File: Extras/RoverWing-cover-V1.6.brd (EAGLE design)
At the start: 81.3 x 81.3 mm, 52 parts, among them J1 HEADER-PH-3PSIDEENTRY, J10 HEADER-PH-6PSIDEENTRY, J13 HEADER-PH-6PSIDEENTRY, J16 FEATHERWING_NODIM, J17 HEADER-PH-6PSIDEENTRY, J5 HEADER-PH-6PSIDEENTRY

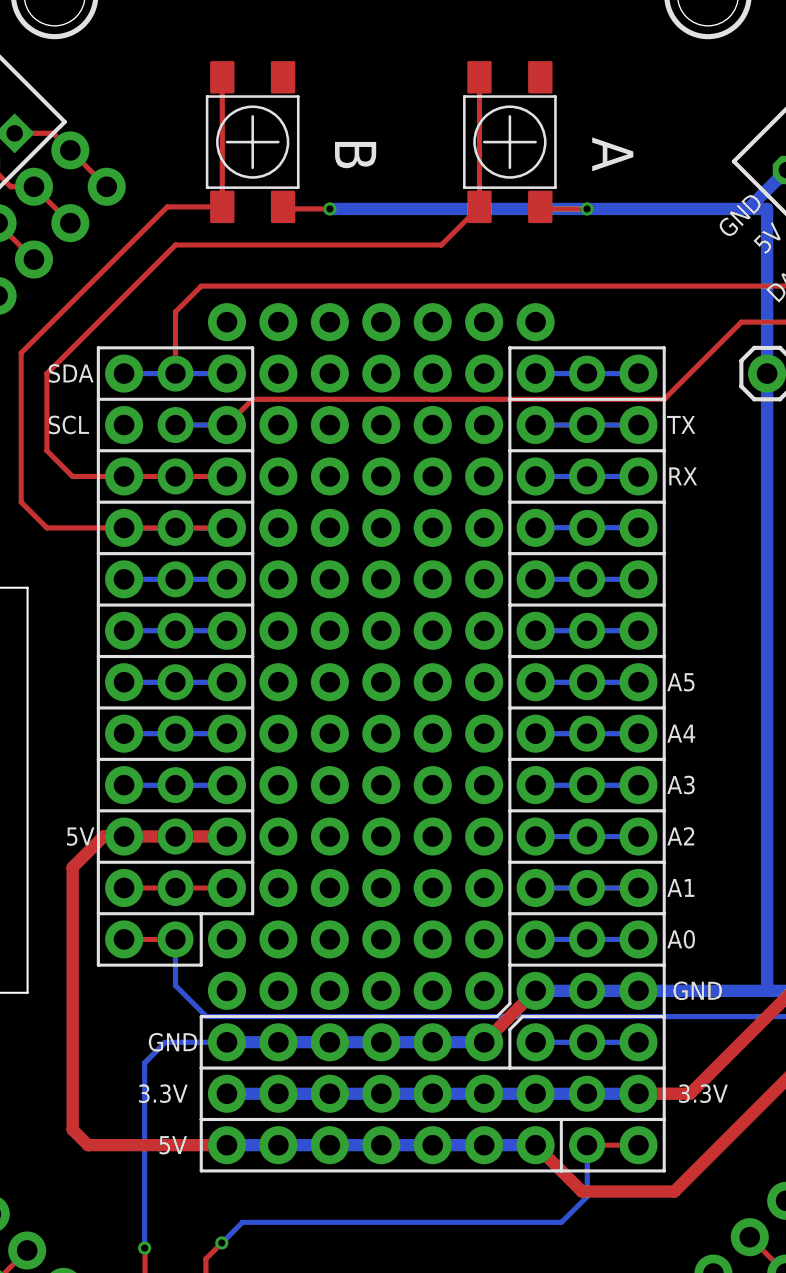
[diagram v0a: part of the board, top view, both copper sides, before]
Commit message: Update RoverWing-cover-V1.6.brd
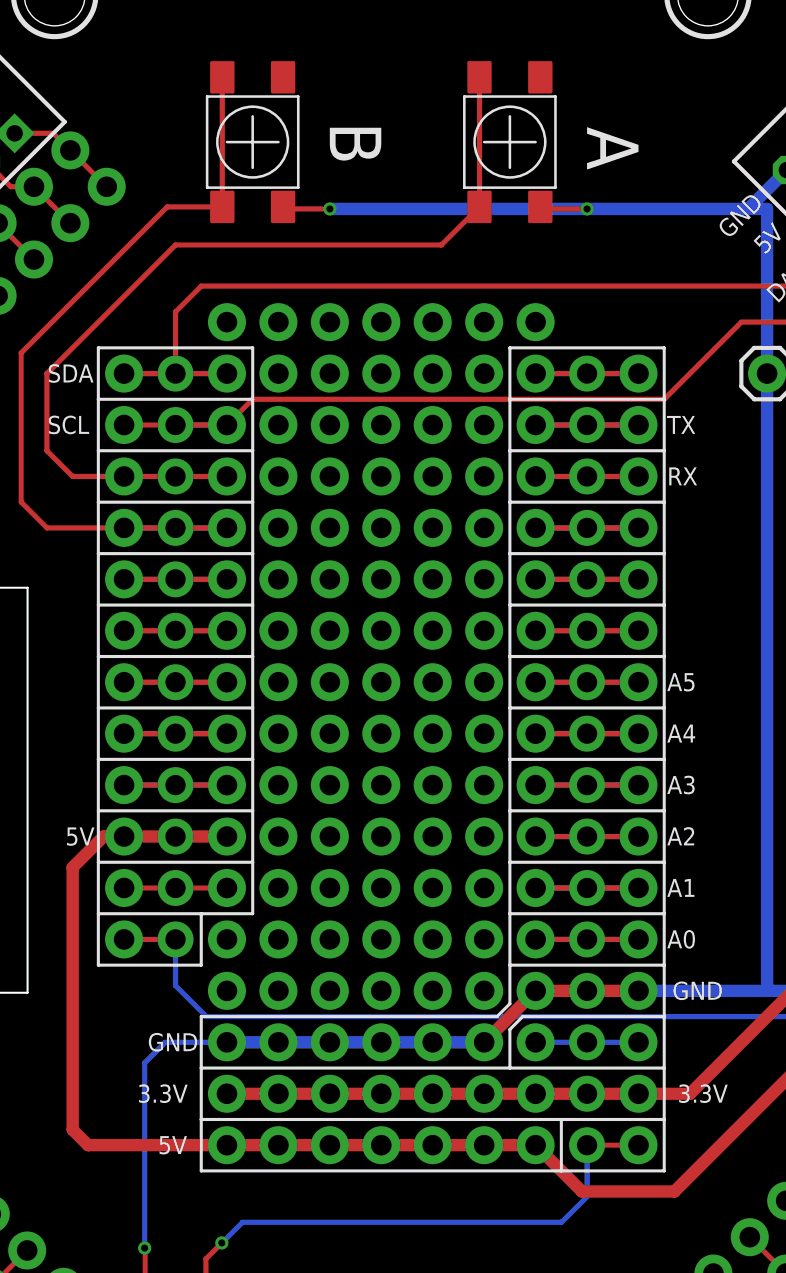
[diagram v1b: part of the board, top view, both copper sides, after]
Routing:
- net TX: track 5.08 -> 10.4 mm
- net SCK: track 5.08 -> 10.2 mm
- net RX: track 5.08 -> 10.2 mm
- net MOSI: track 5.08 -> 10.2 mm
- net MISO: track 5.08 -> 10.2 mm
- net EXTRA: track 5.08 -> 10.2 mm
- net D13: track 5.08 -> 10.2 mm
- net D12: track 5.08 -> 10.2 mm
- net D11: track 5.08 -> 10.2 mm
- net D10: track 5.08 -> 10.2 mm
- net D09: track 5.08 -> 10.2 mm
- net A5: track 5.08 -> 10.2 mm
- net A4: track 5.08 -> 10.2 mm
- net A3: track 5.08 -> 10.2 mm
- net A2: track 5.08 -> 10.2 mm
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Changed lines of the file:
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@@
 <wire x1="6.35" y1="15.24" x2="13.97" y2="15.24" width="0.1524" layer="22"/>
 <wire x1="6.35" y1="17.78" x2="13.97" y2="17.78" width="0.1524" layer="22"/>
-<text x="10.414" y="30.734" size="2.032" layer="25" font="vector" ratio="14" rot="SR270">A</text>
-<text x="-2.286" y="30.734" size="2.032" layer="25" font="vector" ratio="14" rot="SR270">B</text>
+<text x="10.16" y="31.242" size="2.54" layer="25" font="vector" ratio="14" rot="SR270">A</text>
+<text x="-2.54" y="31.496" size="2.54" layer="25" font="vector" ratio="14" rot="SR270">B</text>
 <wire x1="-8.89" y1="-7.62" x2="-8.89" y2="-10.16" width="0.1524" layer="21"/>
 <wire x1="-13.97" y1="-10.16" x2="-8.89" y2="-10.16" width="0.1524" layer="22"/>
@@
 <contactref element="S3" pad="2"/>
 <wire x1="-7.62" y1="-13.97" x2="5.08" y2="-13.97" width="0.6096" layer="16"/>
-<wire x1="7.62" y1="-11.43" x2="12.7" y2="-11.43" width="0.6096" layer="16"/>
 <wire x1="10.16" y1="27.178" x2="-2.54" y2="27.178" width="0.6096" layer="16"/>
 <via x="-2.54" y="27.178" extent="1-16" drill="0.35"/>
@@
 <wire x1="34.685" y1="-1.75" x2="32.484" y2="-1.75" width="0.3048" layer="1"/>
 <wire x1="32.484" y1="-1.75" x2="31.623" y2="-0.889" width="0.3048" layer="1"/>
+<wire x1="7.62" y1="-11.43" x2="12.7" y2="-11.43" width="0.6096" layer="1"/>
 <wire x1="-11.66" y1="-27.28" x2="-11.66" y2="-33.68" width="0" layer="19" extent="1-1"/>
 <wire x1="29.337" y1="-8.509" x2="29.21" y2="-8.509" width="0" layer="19" extent="1-16"/>
@@
 <wire x1="26.543" y1="28.829" x2="22.584209375" y2="28.829" width="0.6096" layer="1"/>
 <wire x1="21.441209375" y1="27.686" x2="22.584209375" y2="28.829" width="0.6096" layer="1"/>
-<wire x1="-7.62" y1="-19.05" x2="7.62" y2="-19.05" width="0.6096" layer="16"/>
 <wire x1="34.544" y1="-14.224" x2="38.862" y2="-9.906" width="0.6096" layer="1"/>
 <wire x1="38.862" y1="-9.906" x2="38.862" y2="-7.62" width="0.6096" layer="1"/>
@@
 <wire x1="36.435" y1="-5.87" x2="36.435" y2="-7.507" width="0.3048" layer="1"/>
 <wire x1="36.435" y1="-7.507" x2="36.322" y2="-7.62" width="0.3048" layer="1"/>
+<wire x1="7.62" y1="-19.05" x2="-7.62" y2="-19.05" width="0.6096" layer="1"/>
 <wire x1="-2.54" y1="-19.05" x2="-5.08" y2="-19.05" width="0" layer="19" extent="1-1"/>
 <wire x1="0" y1="-19.05" x2="-2.54" y2="-19.05" width="0" layer="19" extent="1-1"/>
@@
 <contactref element="J113" pad="7"/>
 <wire x1="10.16" y1="-8.89" x2="7.62" y2="-8.89" width="0.254" layer="16"/>
+<wire x1="7.62" y1="-8.89" x2="12.7" y2="-8.89" width="0.254" layer="1"/>
 </signal>
 <signal name="A1">
@@
 <wire x1="12.7" y1="-6.35" x2="10.16" y2="-6.35" width="0.254" layer="16"/>
 <wire x1="10.16" y1="-6.35" x2="7.62" y2="-6.35" width="0.254" layer="16"/>
+<wire x1="7.62" y1="-6.35" x2="12.7" y2="-6.35" width="0.254" layer="1"/>
 </signal>
 <signal name="A2">
@@
 <wire x1="12.7" y1="-3.81" x2="10.16" y2="-3.81" width="0.254" layer="16"/>
 <wire x1="10.16" y1="-3.81" x2="7.62" y2="-3.81" width="0.254" layer="16"/>
+<wire x1="7.62" y1="-3.81" x2="12.7" y2="-3.81" width="0.254" layer="1"/>
 </signal>
 <signal name="A3">
@@
 <wire x1="12.7" y1="-1.27" x2="10.16" y2="-1.27" width="0.254" layer="16"/>
 <wire x1="10.16" y1="-1.27" x2="7.62" y2="-1.27" width="0.254" layer="16"/>
+<wire x1="7.62" y1="-1.27" x2="12.7" y2="-1.27" width="0.254" layer="1"/>
 </signal>
 <signal name="A4">
@@
 <wire x1="12.7" y1="1.27" x2="10.16" y2="1.27" width="0.254" layer="16"/>
 <wire x1="10.16" y1="1.27" x2="7.62" y2="1.27" width="0.254" layer="16"/>
+<wire x1="7.62" y1="1.27" x2="12.7" y2="1.27" width="0.254" layer="1"/>
 </signal>
 <signal name="A5">
@@
 <wire x1="12.7" y1="3.81" x2="10.16" y2="3.81" width="0.254" layer="16"/>
 <wire x1="10.16" y1="3.81" x2="7.62" y2="3.81" width="0.254" layer="16"/>
+<wire x1="7.62" y1="3.81" x2="12.7" y2="3.81" width="0.254" layer="1"/>
 </signal>
 <signal name="SCK">
@@
 <wire x1="7.62" y1="6.35" x2="10.16" y2="6.35" width="0.254" layer="16"/>
 <wire x1="10.16" y1="6.35" x2="12.7" y2="6.35" width="0.254" layer="16"/>
+<wire x1="7.62" y1="6.35" x2="12.7" y2="6.35" width="0.254" layer="1"/>
 </signal>
 <signal name="MOSI">
@@
 <wire x1="7.62" y1="8.89" x2="10.16" y2="8.89" width="0.254" layer="16"/>
 <wire x1="10.16" y1="8.89" x2="12.7" y2="8.89" width="0.254" layer="16"/>
+<wire x1="7.62" y1="8.89" x2="12.7" y2="8.89" width="0.254" layer="1"/>
 </signal>
 <signal name="MISO">
@@
 <wire x1="7.62" y1="11.43" x2="10.16" y2="11.43" width="0.254" layer="16"/>
 <wire x1="12.7" y1="11.43" x2="10.16" y2="11.43" width="0.254" layer="16"/>
+<wire x1="7.62" y1="11.43" x2="12.7" y2="11.43" width="0.254" layer="1"/>
 </signal>
 <signal name="RX">
@@
 <wire x1="12.7" y1="13.97" x2="10.16" y2="13.97" width="0.254" layer="16"/>
 <wire x1="10.16" y1="13.97" x2="7.62" y2="13.97" width="0.254" layer="16"/>
+<wire x1="7.62" y1="13.97" x2="12.7" y2="13.97" width="0.254" layer="1"/>
 </signal>
 <signal name="TX">
@@
 <wire x1="12.7" y1="16.51" x2="10.16" y2="16.51" width="0.254" layer="16"/>
 <wire x1="10.16" y1="16.51" x2="7.62" y2="16.51" width="0.254" layer="16"/>
+<wire x1="7.62" y1="16.51" x2="12.954" y2="16.51" width="0.254" layer="1"/>
 </signal>
 <signal name="EXTRA">
@@
 <wire x1="10.16" y1="19.05" x2="7.62" y2="19.05" width="0.254" layer="16"/>
 <wire x1="12.7" y1="19.05" x2="10.16" y2="19.05" width="0.254" layer="16"/>
+<wire x1="7.62" y1="19.05" x2="12.7" y2="19.05" width="0.254" layer="1"/>
 </signal>
 <signal name="N$37">
@@
 <wire x1="-12.7" y1="-1.27" x2="-10.16" y2="-1.27" width="0.254" layer="16"/>
 <wire x1="-10.16" y1="-1.27" x2="-7.62" y2="-1.27" width="0.254" layer="16"/>
+<wire x1="-12.7" y1="-1.27" x2="-7.62" y2="-1.27" width="0.254" layer="1"/>
 </signal>
 <signal name="D12">
@@
 <wire x1="-12.7" y1="1.27" x2="-10.16" y2="1.27" width="0.254" layer="16"/>
 <wire x1="-10.16" y1="1.27" x2="-7.62" y2="1.27" width="0.254" layer="16"/>
+<wire x1="-12.7" y1="1.27" x2="-7.62" y2="1.27" width="0.254" layer="1"/>
 </signal>
 <signal name="D11">
@@
 <wire x1="-12.7" y1="3.81" x2="-10.16" y2="3.81" width="0.254" layer="16"/>
 <wire x1="-10.16" y1="3.81" x2="-7.62" y2="3.81" width="0.254" layer="16"/>
+<wire x1="-12.7" y1="3.81" x2="-7.62" y2="3.81" width="0.254" layer="1"/>
 </signal>
 <signal name="D10">
@@
 <wire x1="-12.7" y1="6.35" x2="-10.16" y2="6.35" width="0.254" layer="16"/>
 <wire x1="-10.16" y1="6.35" x2="-7.62" y2="6.35" width="0.254" layer="16"/>
+<wire x1="-12.7" y1="6.35" x2="-7.62" y2="6.35" width="0.254" layer="1"/>
 </signal>
 <signal name="D06">
@@
 <wire x1="-12.7" y1="8.89" x2="-10.16" y2="8.89" width="0.254" layer="16"/>
 <wire x1="-10.16" y1="8.89" x2="-7.62" y2="8.89" width="0.254" layer="16"/>
+<wire x1="-12.7" y1="8.89" x2="-7.62" y2="8.89" width="0.254" layer="1"/>
 </signal>
 <signal name="N$3">
@@
 <wire x1="26.67" y1="19.05" x2="22.352" y2="23.368" width="0.254" layer="1"/>
 <wire x1="-8.89" y1="23.368" x2="22.352" y2="23.368" width="0.254" layer="1"/>
+<wire x1="-12.7" y1="19.05" x2="-7.62" y2="19.05" width="0.254" layer="1"/>
 </signal>
 <signal name="SCL">
@@
 <wire x1="17.78" y1="21.59" x2="21.59" y2="21.59" width="0.254" layer="1"/>
 <wire x1="21.59" y1="21.59" x2="24.13" y2="19.05" width="0.254" layer="1"/>
-<wire x1="-12.7" y1="16.51" x2="-10.16" y2="16.51" width="0" layer="19" extent="1-1"/>
+<wire x1="-12.7" y1="16.51" x2="-7.62" y2="16.51" width="0.254" layer="1"/>
 </signal>
 <signal name="3.3V">
@@
 <contactref element="J116" pad="1"/>
 <contactref element="J2" pad="2"/>
-<wire x1="-7.62" y1="-16.51" x2="12.7" y2="-16.51" width="0.6096" layer="16"/>
 <wire x1="21.59" y1="19.05" x2="21.59" y2="-10.16" width="0.6096" layer="1"/>
 <wire x1="21.59" y1="-10.16" x2="15.24" y2="-16.51" width="0.6096" layer="1"/>
 <wire x1="15.24" y1="-16.51" x2="12.7" y2="-16.51" width="0.6096" layer="1"/>
+<wire x1="-7.62" y1="-16.51" x2="12.7" y2="-16.51" width="0.6096" layer="1"/>
 <wire x1="-2.54" y1="-16.51" x2="-5.08" y2="-16.51" width="0" layer="19" extent="1-1"/>
 <wire x1="0" y1="-16.51" x2="-2.54" y2="-16.51" width="0" layer="19" extent="1-1"/>

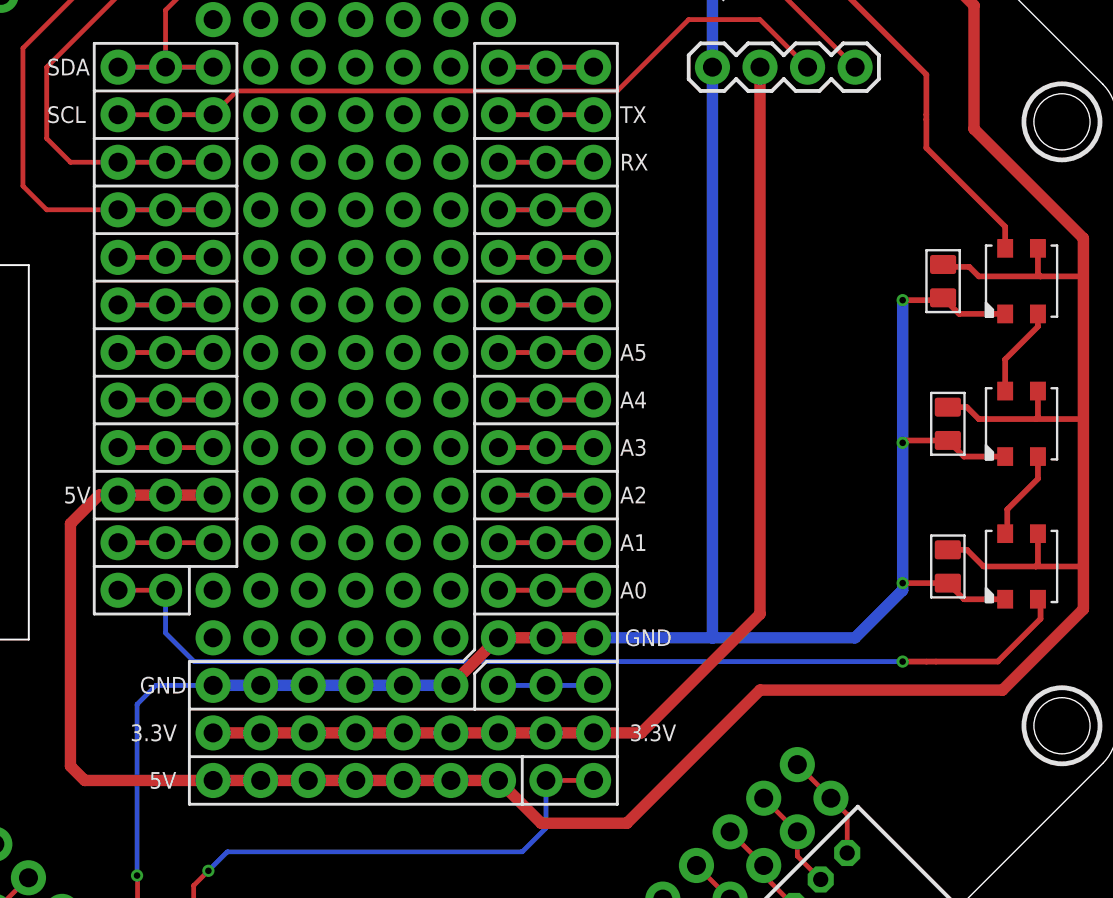
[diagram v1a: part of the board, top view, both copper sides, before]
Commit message: docs update
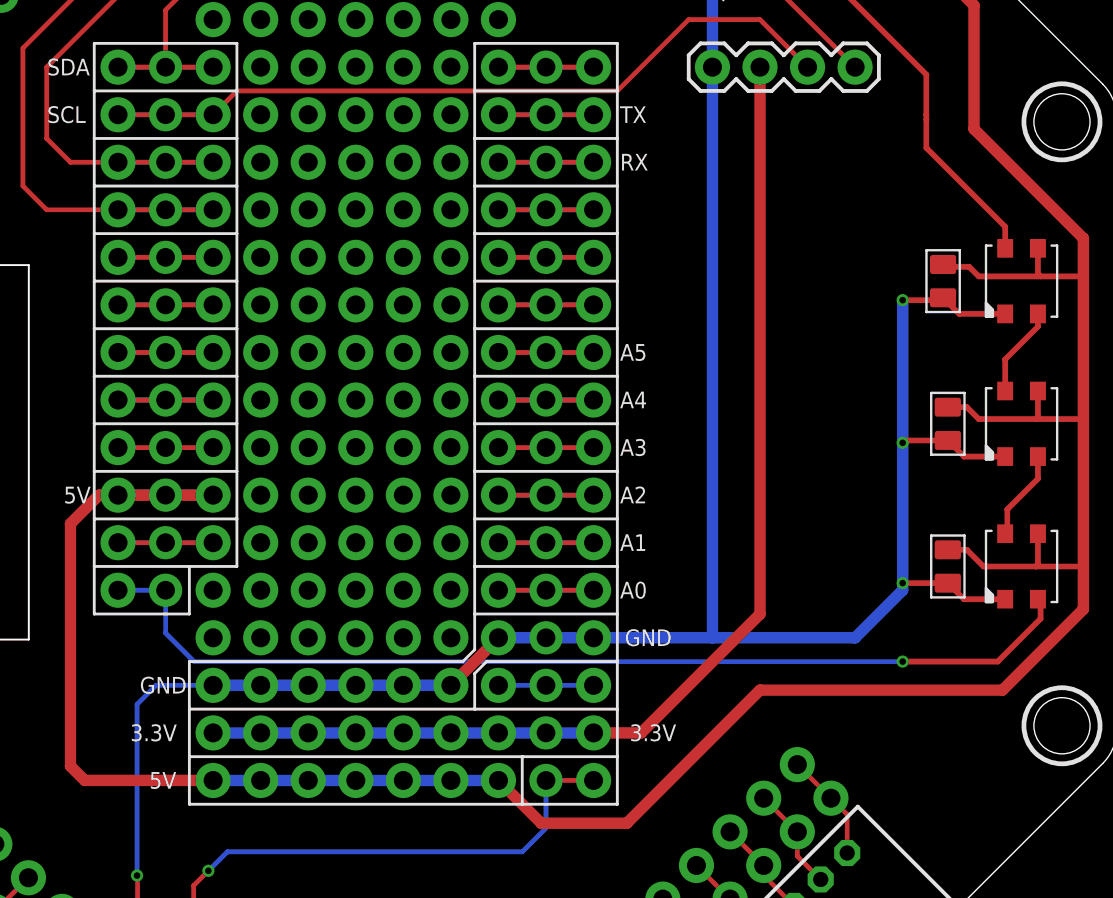
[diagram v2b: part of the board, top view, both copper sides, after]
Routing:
- net 5V: track 158.5 -> 163.6 mm
- net N$37: track 5.08 -> 10.2 mm
- net SCL: track 42.5 -> 45.1 mm
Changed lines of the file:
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@@
 <contactref element="S3" pad="3"/>
 <contactref element="S3" pad="2"/>
-<wire x1="-7.62" y1="-13.97" x2="5.08" y2="-13.97" width="0.6096" layer="16"/>
 <wire x1="10.16" y1="27.178" x2="-2.54" y2="27.178" width="0.6096" layer="16"/>
 <via x="-2.54" y="27.178" extent="1-16" drill="0.35"/>
@@
 <wire x1="34.685" y1="-1.75" x2="32.484" y2="-1.75" width="0.3048" layer="1"/>
 <wire x1="32.484" y1="-1.75" x2="31.623" y2="-0.889" width="0.3048" layer="1"/>
-<wire x1="7.62" y1="-11.43" x2="12.7" y2="-11.43" width="0.6096" layer="1"/>
+<wire x1="-7.62" y1="-13.97" x2="5.08" y2="-13.97" width="0.6096" layer="16"/>
+<wire x1="12.7" y1="-11.43" x2="7.62" y2="-11.43" width="0.6096" layer="16"/>
 <wire x1="-11.66" y1="-27.28" x2="-11.66" y2="-33.68" width="0" layer="19" extent="1-1"/>
 <wire x1="29.337" y1="-8.509" x2="29.21" y2="-8.509" width="0" layer="19" extent="1-16"/>
@@
 <wire x1="0" y1="-13.97" x2="-2.54" y2="-13.97" width="0" layer="19" extent="1-1"/>
 <wire x1="2.54" y1="-13.97" x2="5.08" y2="-13.97" width="0" layer="19" extent="16-16"/>
-<wire x1="10.16" y1="-11.43" x2="7.62" y2="-11.43" width="0" layer="19" extent="1-1"/>
+<wire x1="10.16" y1="-11.43" x2="12.7" y2="-11.43" width="0" layer="19" extent="1-1"/>
 <wire x1="7.85" y1="33.68" x2="7.85" y2="27.28" width="0" layer="19" extent="1-1"/>
 <wire x1="-4.85" y1="33.68" x2="-4.85" y2="27.28" width="0" layer="19" extent="1-1"/>
@@
 <wire x1="36.435" y1="-5.87" x2="36.435" y2="-7.507" width="0.3048" layer="1"/>
 <wire x1="36.435" y1="-7.507" x2="36.322" y2="-7.62" width="0.3048" layer="1"/>
-<wire x1="7.62" y1="-19.05" x2="-7.62" y2="-19.05" width="0.6096" layer="1"/>
+<wire x1="-7.62" y1="-19.05" x2="7.62" y2="-19.05" width="0.6096" layer="16"/>
+<wire x1="-12.7" y1="-3.81" x2="-7.62" y2="-3.81" width="0.6096" layer="16"/>
 <wire x1="-2.54" y1="-19.05" x2="-5.08" y2="-19.05" width="0" layer="19" extent="1-1"/>
 <wire x1="0" y1="-19.05" x2="-2.54" y2="-19.05" width="0" layer="19" extent="1-1"/>
@@
 <contactref element="J112" pad="1"/>
 <wire x1="-10.16" y1="-6.35" x2="-7.62" y2="-6.35" width="0.254" layer="1"/>
+<wire x1="-12.7" y1="-6.35" x2="-7.62" y2="-6.35" width="0.254" layer="16"/>
 </signal>
 <signal name="D13">
@@
 <wire x1="21.59" y1="21.59" x2="24.13" y2="19.05" width="0.254" layer="1"/>
 <wire x1="-12.7" y1="16.51" x2="-7.62" y2="16.51" width="0.254" layer="1"/>
+<wire x1="-12.7" y1="16.51" x2="-10.16" y2="16.51" width="0.254" layer="16"/>
 </signal>
 <signal name="3.3V">
@@
 <wire x1="21.59" y1="-10.16" x2="15.24" y2="-16.51" width="0.6096" layer="1"/>
 <wire x1="15.24" y1="-16.51" x2="12.7" y2="-16.51" width="0.6096" layer="1"/>
-<wire x1="-7.62" y1="-16.51" x2="12.7" y2="-16.51" width="0.6096" layer="1"/>
+<wire x1="-7.62" y1="-16.51" x2="12.7" y2="-16.51" width="0.6096" layer="16"/>
 <wire x1="-2.54" y1="-16.51" x2="-5.08" y2="-16.51" width="0" layer="19" extent="1-1"/>
 <wire x1="0" y1="-16.51" x2="-2.54" y2="-16.51" width="0" layer="19" extent="1-1"/>
@@
 <contactref element="J16" pad="28"/>
 <contactref element="J3" pad="1"/>
-<wire x1="-12.7" y1="-8.89" x2="-10.16" y2="-8.89" width="0.254" layer="1"/>
 <wire x1="-8.636" y1="-12.7" x2="-10.16" y2="-11.176" width="0.254" layer="16"/>
 <wire x1="-10.16" y1="-8.89" x2="-10.16" y2="-11.176" width="0.254" layer="16"/>
 <wire x1="-8.636" y1="-12.7" x2="29.21" y2="-12.7" width="0.254" layer="16"/>
 <via x="29.21" y="-12.7" extent="1-16" drill="0.35"/>
-<wire x1="29.21" y1="-12.7" x2="30.48" y2="-12.7" width="0.3048" layer="1"/>
-<wire x1="30.48" y1="-12.7" x2="30.988" y2="-12.7" width="0.3048" layer="1"/>
-<wire x1="30.988" y1="-12.7" x2="34.29" y2="-12.7" width="0.3048" layer="1"/>
+<wire x1="29.21" y1="-12.7" x2="34.29" y2="-12.7" width="0.3048" layer="1"/>
 <wire x1="34.29" y1="-12.7" x2="36.576" y2="-10.414" width="0.3048" layer="1"/>
 <wire x1="36.576" y1="-10.414" x2="36.576" y2="-9.511" width="0.3048" layer="1"/>
 <wire x1="36.576" y1="-9.511" x2="36.435" y2="-9.37" width="0.3048" layer="1"/>
+<wire x1="-12.7" y1="-8.89" x2="-10.16" y2="-8.89" width="0.254" layer="16"/>
 </signal>
 <signal name="N$2">
